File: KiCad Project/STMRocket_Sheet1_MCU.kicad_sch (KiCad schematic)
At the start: 22 parts, among them U1 STM32F103C8T6, Y1 ECS-2520MV-160-CN-TR

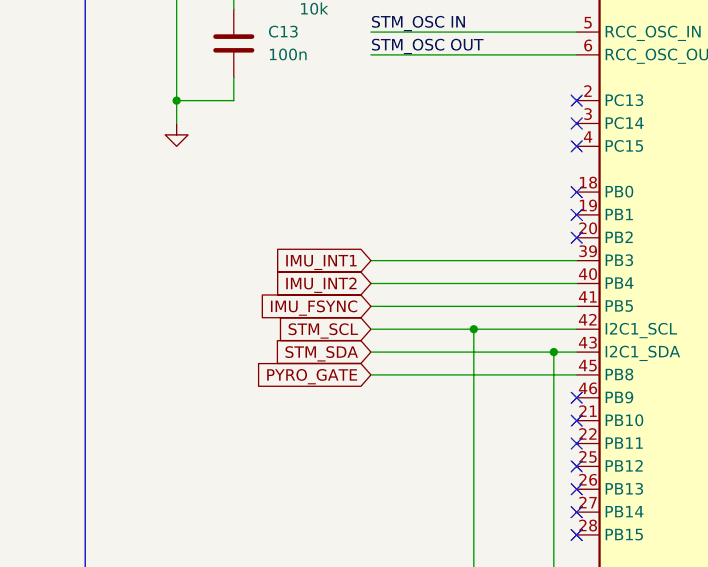
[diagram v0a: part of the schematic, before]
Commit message: PCB update
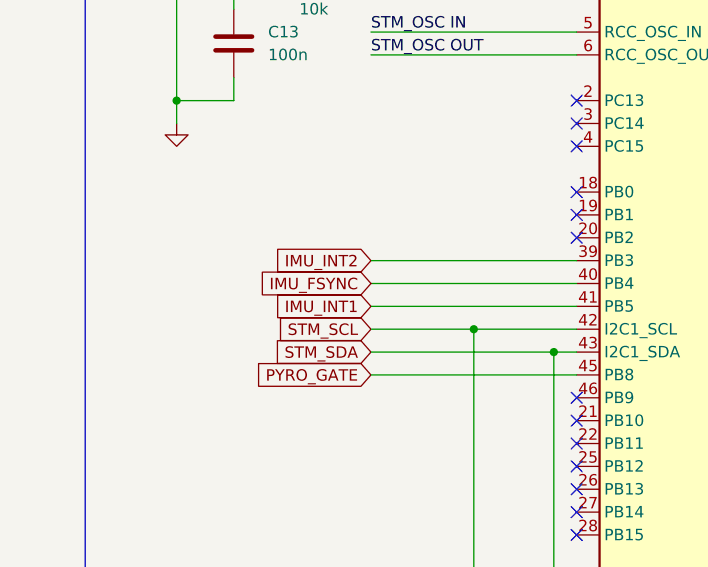
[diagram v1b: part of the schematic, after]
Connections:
- net IMU_FSYNC: now also U1.40 (PB4); no longer U1.41 (PB5)
- net IMU_INT1: now also U1.41 (PB5); no longer U1.39 (PB3)
- net IMU_INT2: now also U1.39 (PB3); no longer U1.40 (PB4)

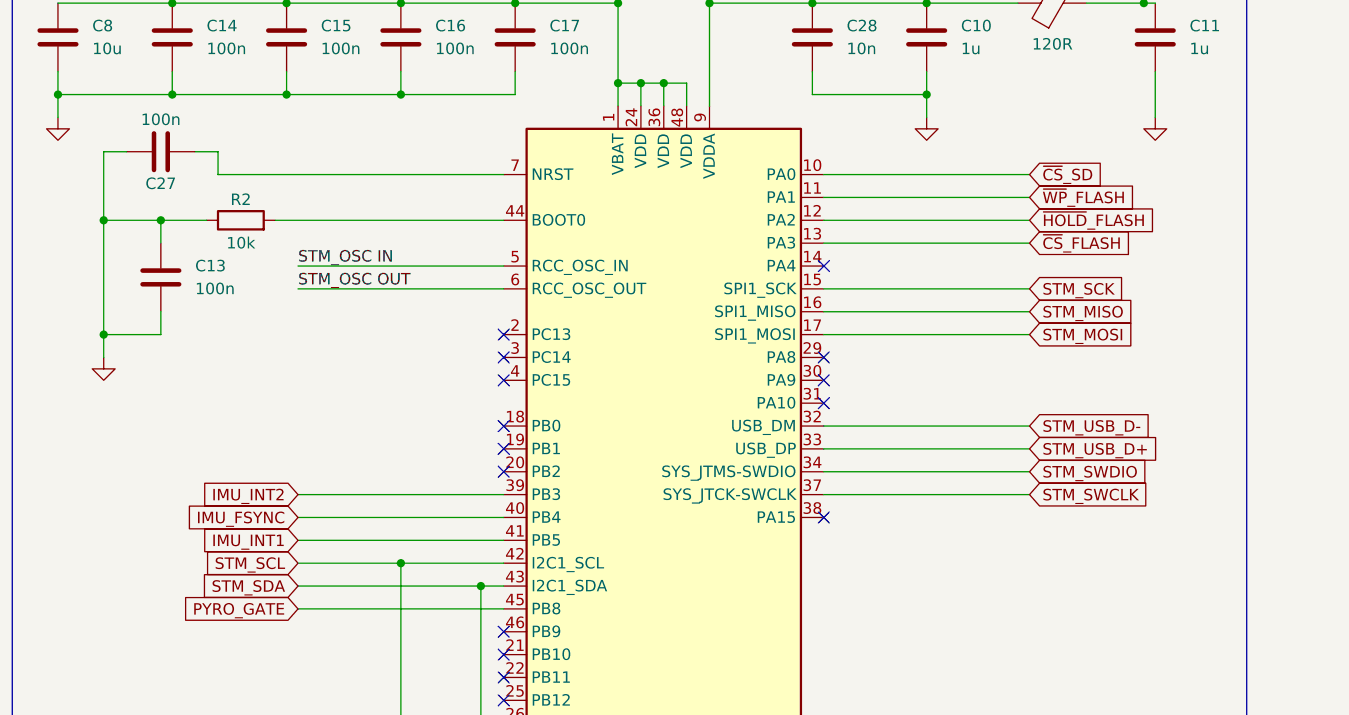
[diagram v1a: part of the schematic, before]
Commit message: finished pcb
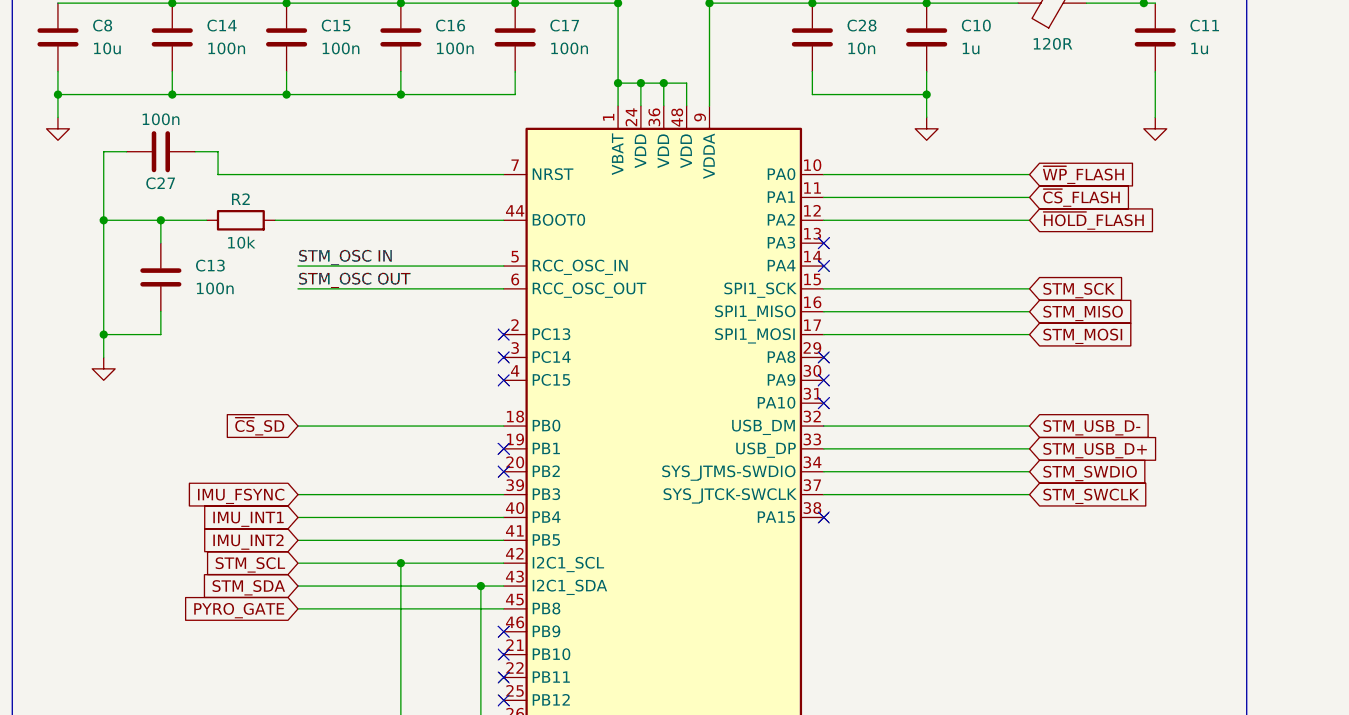
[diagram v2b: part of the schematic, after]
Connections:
- net IMU_FSYNC: now also U1.39 (PB3); no longer U1.40 (PB4)
- net IMU_INT1: now also U1.40 (PB4); no longer U1.41 (PB5)
- net IMU_INT2: now also U1.41 (PB5); no longer U1.39 (PB3)
- net ~{CS}_FLASH: now also U1.11 (PA1); no longer U1.13 (PA3)
- net ~{CS}_SD: now also U1.18 (PB0); no longer U1.10 (PA0)
- net ~{WP}_FLASH: now also U1.10 (PA0); no longer U1.11 (PA1)
